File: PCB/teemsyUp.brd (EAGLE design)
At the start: 80 x 152.1 mm, 22 parts, among them K2 D2F-5, K3 D2F-5, K4 D2F-5, K5 D2F-5

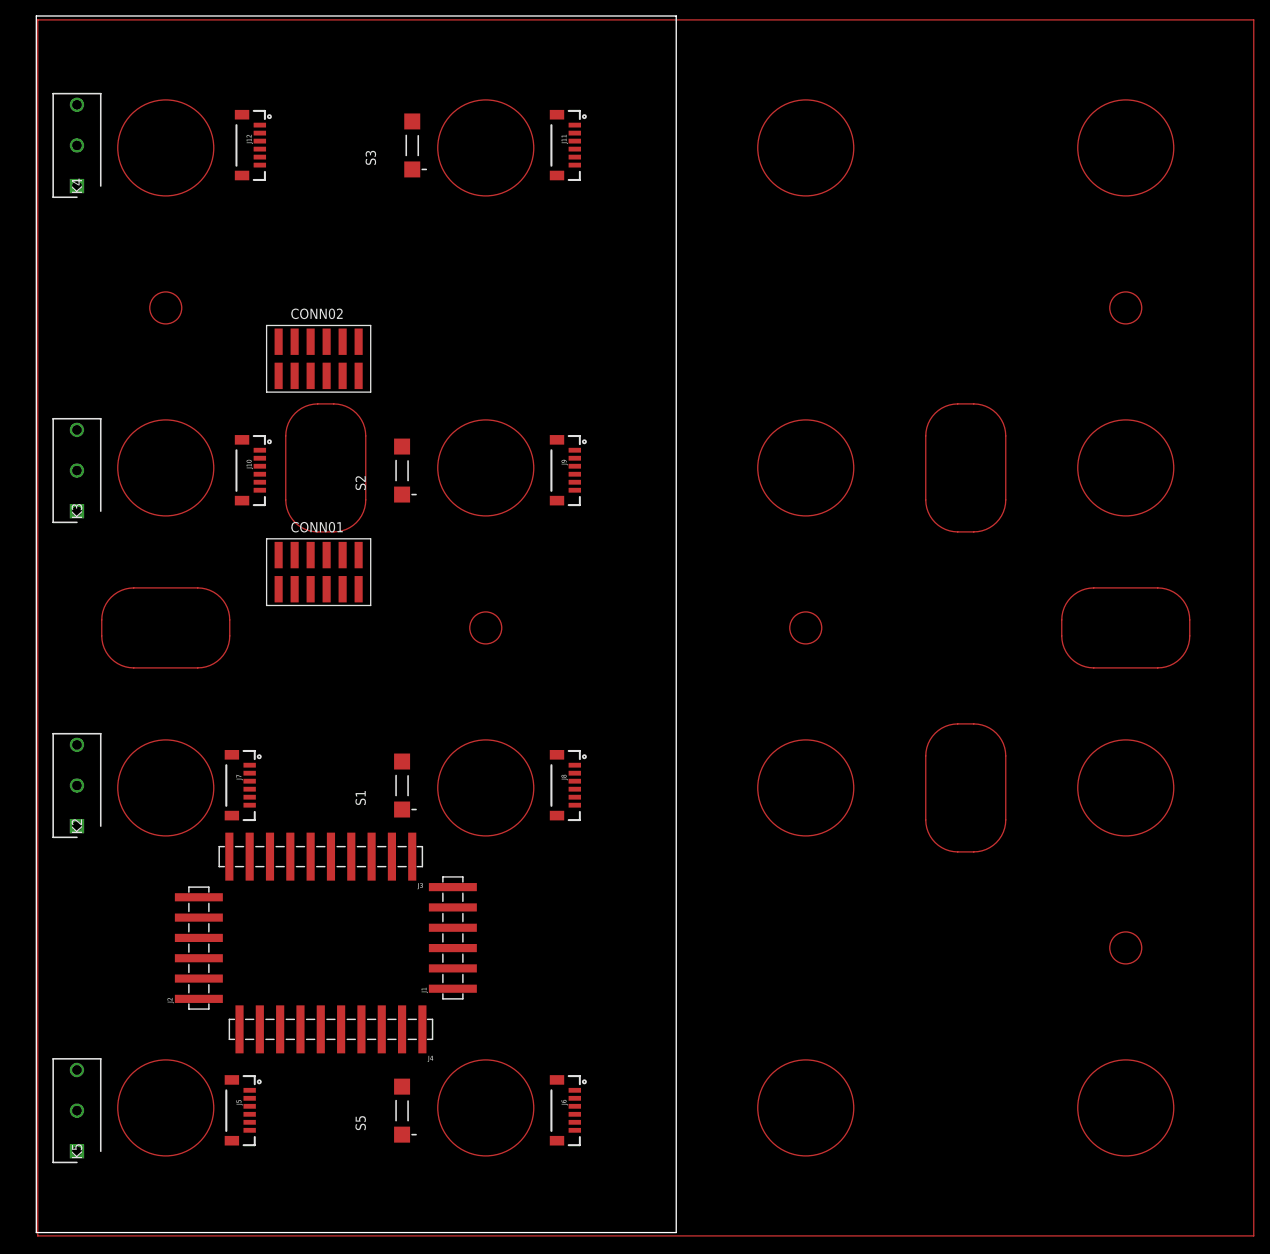
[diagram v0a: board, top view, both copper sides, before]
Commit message: CAN Bus
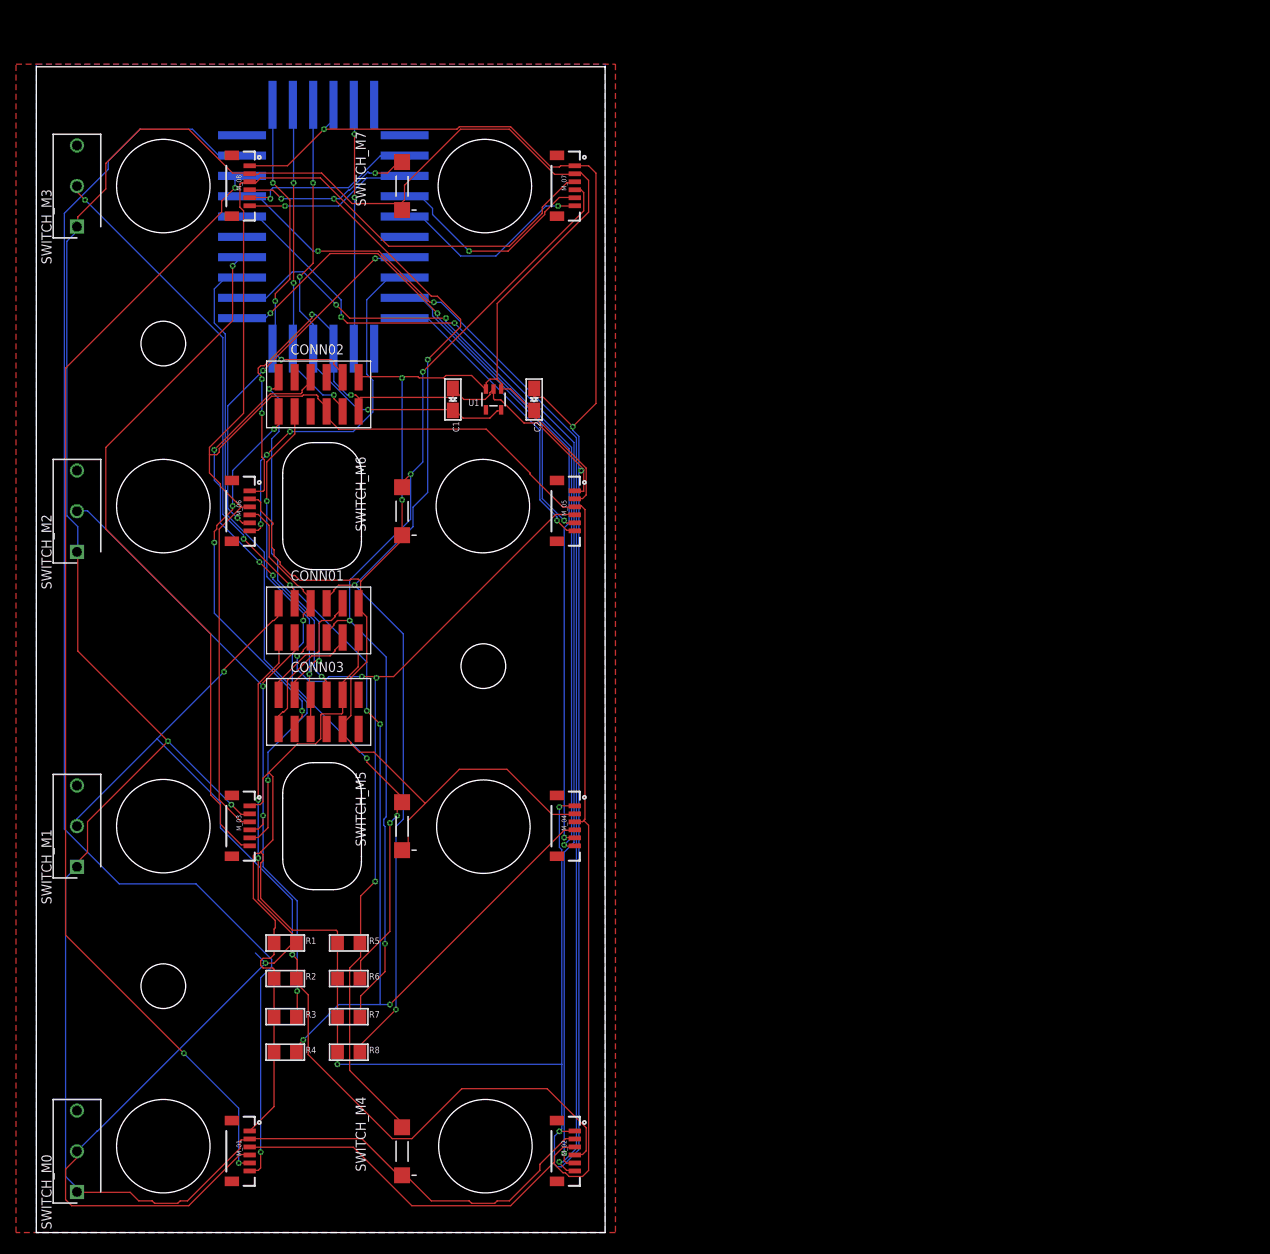
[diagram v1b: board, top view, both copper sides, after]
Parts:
- removed J10, J11, J12, J5, J6, J7, J8, J9: (no value), SparkFun-Connectors:1X06-1MM
- removed K2, K3, K4, K5: D2F-5, D2F-5:SHDR3W100P0X508_1X3_1280X580X5
- removed S1, S2, S3, S5: DTSM-3, switch-tact:DTSM-3
- added C1, C2: (no value), microbuilder:EIA3216-18/A-R
- added CONN03: TMMH-105-12, TMMH-105-XX-XX-DV:TMMH-105-12
- added M_01, M_02, M_03, M_04, M_05, M_06, M_07, M_08: (no value), SparkFun-Connectors:1X06-1MM
- added R1, R2, R3, R4, R5, R6, R7, R8: (no value), microbuilder:1206
- added SWITCH_M0, SWITCH_M1, SWITCH_M2, SWITCH_M3: D2F-5, D2F-5:SHDR3W100P0X508_1X3_1280X580X5
- added SWITCH_M4, SWITCH_M5, SWITCH_M6, SWITCH_M7: DTSM-3, switch-tact:DTSM-3
- added U1: (no value), microbuilder:SOT23-5
- moved J1 110.9 mm to (42.2, 141.0), flipped to the bottom, turned to 0 degrees
- moved J4 88.9 mm to (46.0, 114.3), flipped to the bottom, turned to 90 degrees
- moved J2 84.2 mm to (42.2, 110.5), flipped to the bottom, turned to 0 degrees
- moved J3 70.6 mm to (25.7, 114.3), flipped to the bottom, turned to 90 degrees
- moved CONN01 6.03 mm to (35.6, 76.5)
- moved CONN02 4.44 mm to (35.6, 104.8)
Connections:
- removed net MUX_SCL: J1.6, J2.6
- removed net MUX_SDA: J1.5, J2.5
- removed net N$1: S1.1
- removed net N$10: S2.1
- removed net N$11: S2.2
- removed net N$13: S3.1
- removed net N$14: S5.1
- removed net N$15: S5.2
- removed net N$20: K2.1
- removed net N$21: K2.2
- removed net N$23: K3.2
- removed net N$24: K4.1
- removed net N$25: K4.2
- removed net N$26: K5.1
- removed net N$27: K5.2
- removed net N$7: S1.2
- new net I2CS_0: J3.9, M_01.6
- new net I2CS_1: J3.8, M_01.5
- new net I2CS_10: J4.3, M_06.6
- new net I2CS_11: J4.4, M_06.5
- new net I2CS_12: J4.6, M_07.6
- new net I2CS_13: J4.7, M_07.5
- new net I2CS_14: J4.8, M_08.6
- new net I2CS_15: J4.9, M_08.5
- new net I2CS_2: J3.7, M_02.6
- new net I2CS_3: J3.6, M_02.5
- new net I2CS_4: J3.4, M_03.6
- new net I2CS_5: J3.3, M_03.5
- new net I2CS_6: J3.2, M_04.6
- new net I2CS_7: J3.1, M_04.5
- new net I2CS_8: J4.1, M_05.6
- new net I2CS_9: J4.2, M_05.5
- net 3.3V: now also C1.+, U1.5
- net GND_MCU: now also C1.-, C2.-, CONN03.10, M_01.1, M_02.1, M_03.1, M_04.1, M_05.1, M_06.1, M_07.1, M_08.1, R1.1, R2.1, R3.1, R4.1, R5.1, R6.1, R7.1, R8.1, U1.2
- net I2CM_0: now also M_01.4, R1.2, SWITCH_M0.2; no longer J3.9
- net I2CM_1: now also M_02.4, R2.2, SWITCH_M1.2; no longer J3.8
- net I2CM_10: now also CONN03.3; no longer J4.3
- net I2CM_11: now also CONN03.4; no longer J4.4
- net I2CM_12: now also CONN03.5, CONN03.6; no longer J4.6
- net I2CM_13: no longer J4.7
- net I2CM_14: now also CONN03.7; no longer J4.8
- net I2CM_15: now also CONN03.8; no longer J4.9
- net I2CM_2: now also M_03.4, R3.2, SWITCH_M2.2; no longer J3.7
- net I2CM_3: now also M_04.4, R4.2, SWITCH_M3.2; no longer J3.6
- net I2CM_4: now also M_05.4, R5.2, SWITCH_M4.2; no longer J3.4
- net I2CM_5: now also M_06.4, R6.2, SWITCH_M5.2; no longer J3.3
- net I2CM_6: now also M_07.4, R7.2, SWITCH_M6.2; no longer J3.2
- net I2CM_7: now also M_08.4, R8.2, SWITCH_M7.2; no longer J3.1
- net I2CM_8: now also CONN03.1; no longer J4.1
- net I2CM_9: now also CONN03.2; no longer J4.2
- net N$12: now also CONN03.11; no longer S3.2
- net N$16: now also SWITCH_M3.3; no longer K5.3
- net N$17: now also SWITCH_M2.3; no longer K4.3
- net N$18: now also SWITCH_M1.3; no longer K3.3
- net N$19: now also SWITCH_M0.3; no longer K2.3
- net N$22: now also CONN03.12; no longer K3.1
- net NEO_PIXEL: now also M_01.3, M_02.3, M_03.3, M_04.3, M_05.3, M_06.3, M_07.3, M_08.3
- net S_SCL: now also J1.6, J2.6
- net S_SDA: now also J1.5, J2.5
- net VCC_MCU: now also C2.+, CONN03.9, M_01.2, M_02.2, M_03.2, M_04.2, M_05.2, M_06.2, M_07.2, M_08.2, SWITCH_M0.1, SWITCH_M1.1, SWITCH_M2.1, SWITCH_M3.1, SWITCH_M4.1, SWITCH_M5.1, SWITCH_M6.1, SWITCH_M7.1, U1.1, U1.3
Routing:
- net N$2: track 608.0 -> 0.00 mm
- net VCC_MCU: track 0.00 -> 490.4 mm, vias 0 -> 4
- net GND_MCU: track 0.00 -> 463.4 mm, vias 0 -> 10
- net NEO_PIXEL: track 0.00 -> 331.5 mm
- net I2CM_3: track 0.00 -> 167.3 mm, vias 0 -> 7
- net I2CS_0: track 0.00 -> 166.4 mm, vias 0 -> 1
- net I2CM_7: track 0.00 -> 150.4 mm, vias 0 -> 6
- net I2CS_2: track 0.00 -> 148.5 mm, vias 0 -> 3
- net I2CS_3: track 0.00 -> 146.2 mm, vias 0 -> 3
- net I2CS_1: track 0.00 -> 143.1 mm, vias 0 -> 3
- net I2CM_1: track 0.00 -> 134.1 mm, vias 0 -> 2
- net I2CM_6: track 0.00 -> 126.0 mm, vias 0 -> 4
- net I2CM_0: track 0.00 -> 114.5 mm, vias 0 -> 3
- net I2CM_4: track 0.00 -> 109.3 mm, vias 0 -> 4
- net I2CS_7: track 0.00 -> 104.8 mm, vias 0 -> 3
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- added copper zone on layer 1, net GND_MCU
- added copper zone on layer 16, net GND_MCU
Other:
- board size 80 x 152.1 mm -> 71.1 x 145.7 mm
